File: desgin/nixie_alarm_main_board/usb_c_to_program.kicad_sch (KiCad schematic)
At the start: 3 parts, among them J3 USB_C_Receptacle_USB2.0_16P

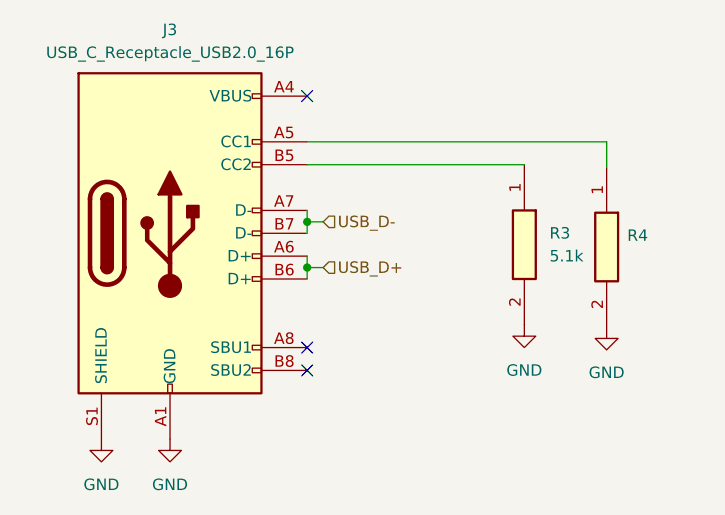
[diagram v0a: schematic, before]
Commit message: filter caps
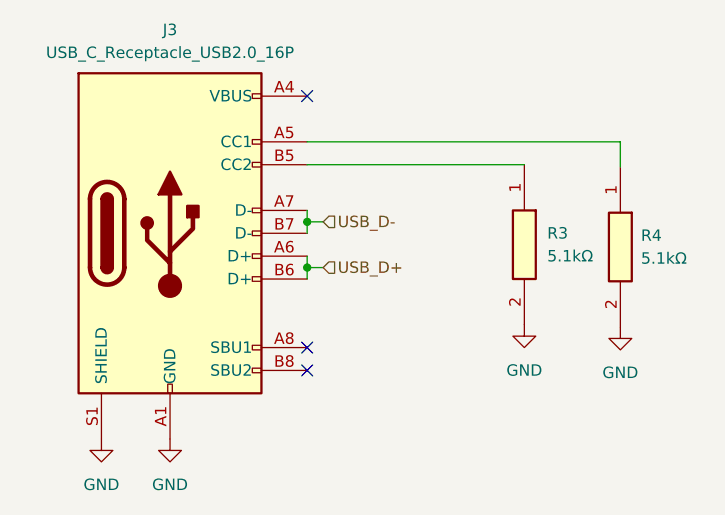
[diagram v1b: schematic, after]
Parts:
- R3, R4: value 5.1k -> 5.1kΩ; footprint ERJUP6 -> RESC2012X60N
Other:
- moved on the sheet: R4
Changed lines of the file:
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@@
 	(wire
 		(pts
-			(xy 146.05 82.55) (xy 179.324 82.55)
+			(xy 146.05 82.55) (xy 180.848 82.55)
 		)
 		(stroke
@@
 	(wire
 		(pts
-			(xy 179.324 82.55) (xy 179.324 85.344)
+			(xy 180.848 82.55) (xy 180.848 85.344)
 		)
 		(stroke
@@
 	(symbol
 		(lib_id "power:GND")
-		(at 179.324 103.124 0)
+		(at 180.848 103.124 0)
 		(unit 1)
 		(exclude_from_sim no)
@@
 		(fields_autoplaced yes)
 		(property "Reference" "#PWR013"
-			(at 179.324 109.474 0)
+			(at 180.848 109.474 0)
 			(effects
 				(font
@@
 		)
 		(property "Value" "GND"
-			(at 179.324 108.204 0)
+			(at 180.848 108.204 0)
 			(effects
 				(font
@@
 		)
 		(property "Footprint" ""
-			(at 179.324 103.124 0)
+			(at 180.848 103.124 0)
 			(effects
 				(font
@@
 		)
 		(property "Datasheet" ""
-			(at 179.324 103.124 0)
+			(at 180.848 103.124 0)
 			(effects
 				(font
@@
 		)
 		(property "Description" "Power symbol creates a global label with name \"GND\" , ground"
-			(at 179.324 103.124 0)
+			(at 180.848 103.124 0)
 			(effects
 				(font
@@
 		(fields_autoplaced yes)
 		(property "Reference" "R3"
-			(at 172.974 92.7099 90)
+			(at 172.72 92.7099 90)
 			(effects
 				(font
@@
 			)
 		)
-		(property "Value" "5.1k"
-			(at 172.974 95.2499 90)
+		(property "Value" "5.1kΩ"
+			(at 172.72 95.2499 90)
 			(effects
 				(font
@@
 			)
 		)
-		(property "Footprint" "ERJUP6"
+		(property "Footprint" "RESC2012X60N"
 			(at 73.99 99.06 0)
 			(effects
@@
 	(symbol
 		(lib_id "SamacSys_Parts:ERJ-UP6D5101V")
-		(at 179.324 85.344 270)
+		(at 180.848 85.344 270)
 		(unit 1)
 		(exclude_from_sim no)
@@
 		(fields_autoplaced yes)
 		(property "Reference" "R4"
-			(at 181.61 92.9639 90)
+			(at 183.134 92.9639 90)
 			(effects
 				(font
@@
 			)
 		)
-		(property "Value" "5.1k"
-			(at 181.61 95.5039 90)
+		(property "Value" "5.1kΩ"
+			(at 183.134 95.5039 90)
 			(effects
 				(font
@@
 				)
 				(justify left)
-				(hide yes)
-			)
-		)
-		(property "Footprint" "ERJUP6"
-			(at 83.134 99.314 0)
+			)
+		)
+		(property "Footprint" "RESC2012X60N"
+			(at 84.658 99.314 0)
 			(effects
 				(font
@@
 		)
 		(property "Datasheet" "https://industrial.panasonic.com/cdbs/www-data/pdf/RDP0000/AOA0000C337.pdf"
-			(at -16.866 99.314 0)
+			(at -15.342 99.314 0)
 			(effects
 				(font
@@
 		)
 		(property "Description" "Anti-Sulfurated Thick Film Chip Resistors/ Anti-Surge Type, Power Rating (W): 0.5, Chip Size (LxW(EIA)) (mm): 2.0 x 1.25 (EIA:0805), Resistance Values (?): 5100, Resistance Tolerance (%): 0.5, T.C.R (?102/K): ?100"
-			(at 179.324 85.344 0)
+			(at 180.848 85.344 0)
 			(effects
 				(font
@@
 		)
 		(property "Height" "0.7"
-			(at -216.866 99.314 0)
+			(at -215.342 99.314 0)
 			(effects
 				(font
@@
 		)
 		(property "Mouser Part Number" "667-ERJ-UP6D5101V"
-			(at -316.866 99.314 0)
+			(at -315.342 99.314 0)
 			(effects
 				(font
@@
 		)
 		(property "Mouser Price/Stock" "https://www.mouser.co.uk/ProductDetail/Panasonic/ERJ-UP6D5101V?qs=ZcfC38r4Pouz7%2FLHthUDHQ%3D%3D"
-			(at -416.866 99.314 0)
+			(at -415.342 99.314 0)
 			(effects
 				(font
@@
 		)
 		(property "Manufacturer_Name" "Panasonic"
-			(at -516.866 99.314 0)
+			(at -515.342 99.314 0)
 			(effects
 				(font
@@
 		)
 		(property "Manufacturer_Part_Number" "ERJ-UP6D5101V"
-			(at -616.866 99.314 0)
-			(effects
-				(font
+			(at -615.342 99.314 0)
+			(effects
+				(font
